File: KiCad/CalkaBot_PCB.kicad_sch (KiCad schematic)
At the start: 36 parts, among them J1 Conn_01x03_Pin, J2 Conn_01x03_Pin, J3 Conn_01x03_Pin, J4 Conn_01x02_Pin, J5 MOTOR3, J6 StartModule, M1 Motor_Right, M2 Motor_Left, Q1 KTIR0711S, Q2 KTIR0711S, Q3 IRLL014NTRPBF, SW1 SW_DIP_x04, U1 L78M05CDT-TR

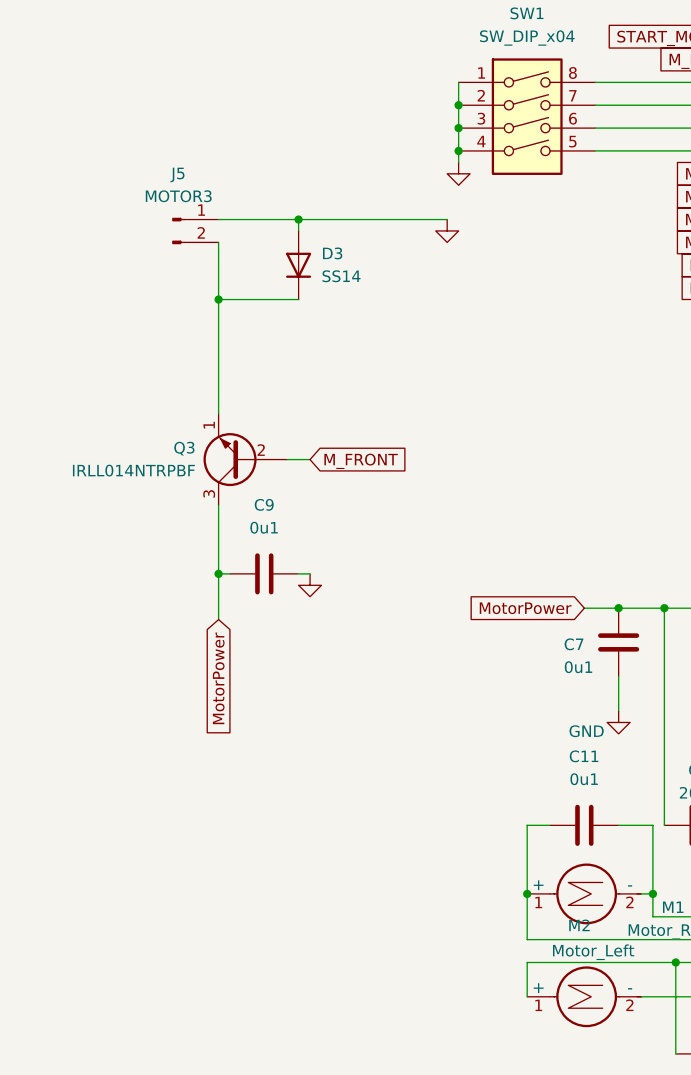
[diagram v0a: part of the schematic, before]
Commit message: working on soft and 2nd version of board
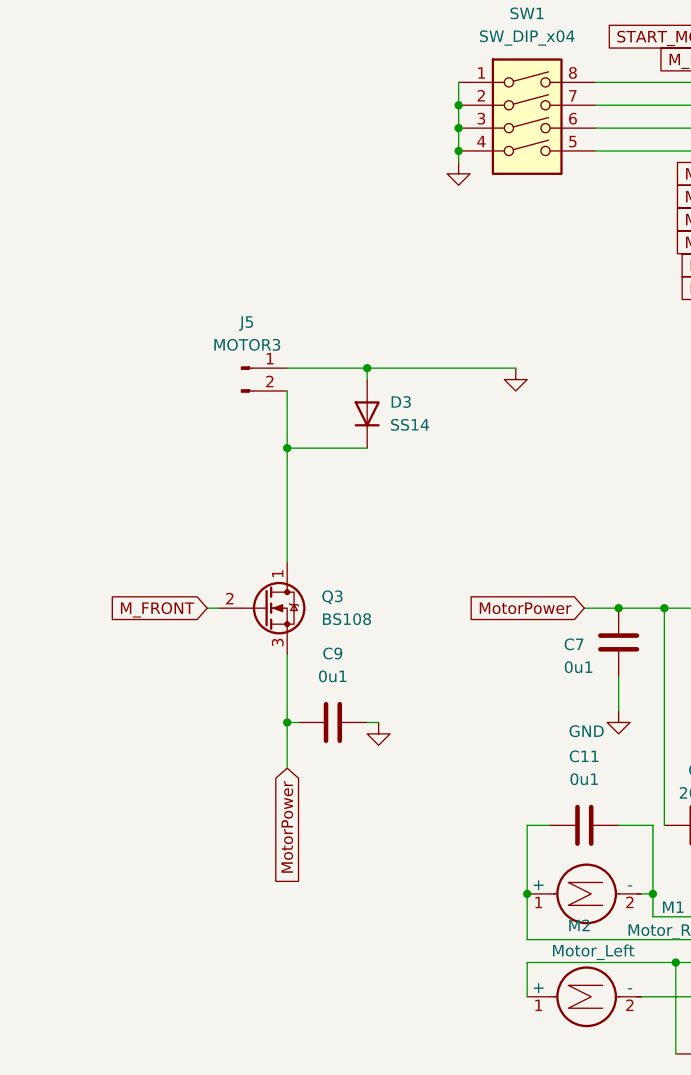
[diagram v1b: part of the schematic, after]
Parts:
- removed Q3: IRLL014NTRPBF, Package_TO_SOT_SMD:SOT-223, symbol Transistor_BJT:BC107
- added Q3: BS108, Package_TO_SOT_THT:TO-92_Inline, symbol Transistor_FET:BS108
- CR1: footprint Package_SO:SO-20-1EP_7.52x12.825mm_P1.27mm_EP6.045x12.09mm_Mask3.56x4.47mm_ThermalVias -> CalkaBot3k0:PowerSO-20
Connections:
- net +7.5V: now also Q3.3 (S)
- net M_FRONT: now also Q3.2 (G)
- net at D3.1 (K), J5.2 (Pin_2): now also Q3.1 (D)
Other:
- moved on the sheet: C9, D3, J5
